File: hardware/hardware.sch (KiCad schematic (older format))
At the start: 39 parts, among them J1 USB_B_Micro, J2 Breakout, Q1 FS8205, U1 DW01+G, U2 TP4056, U3 USBLC6-2, U4 LM317A, U5 PIC18F45K50_QFP

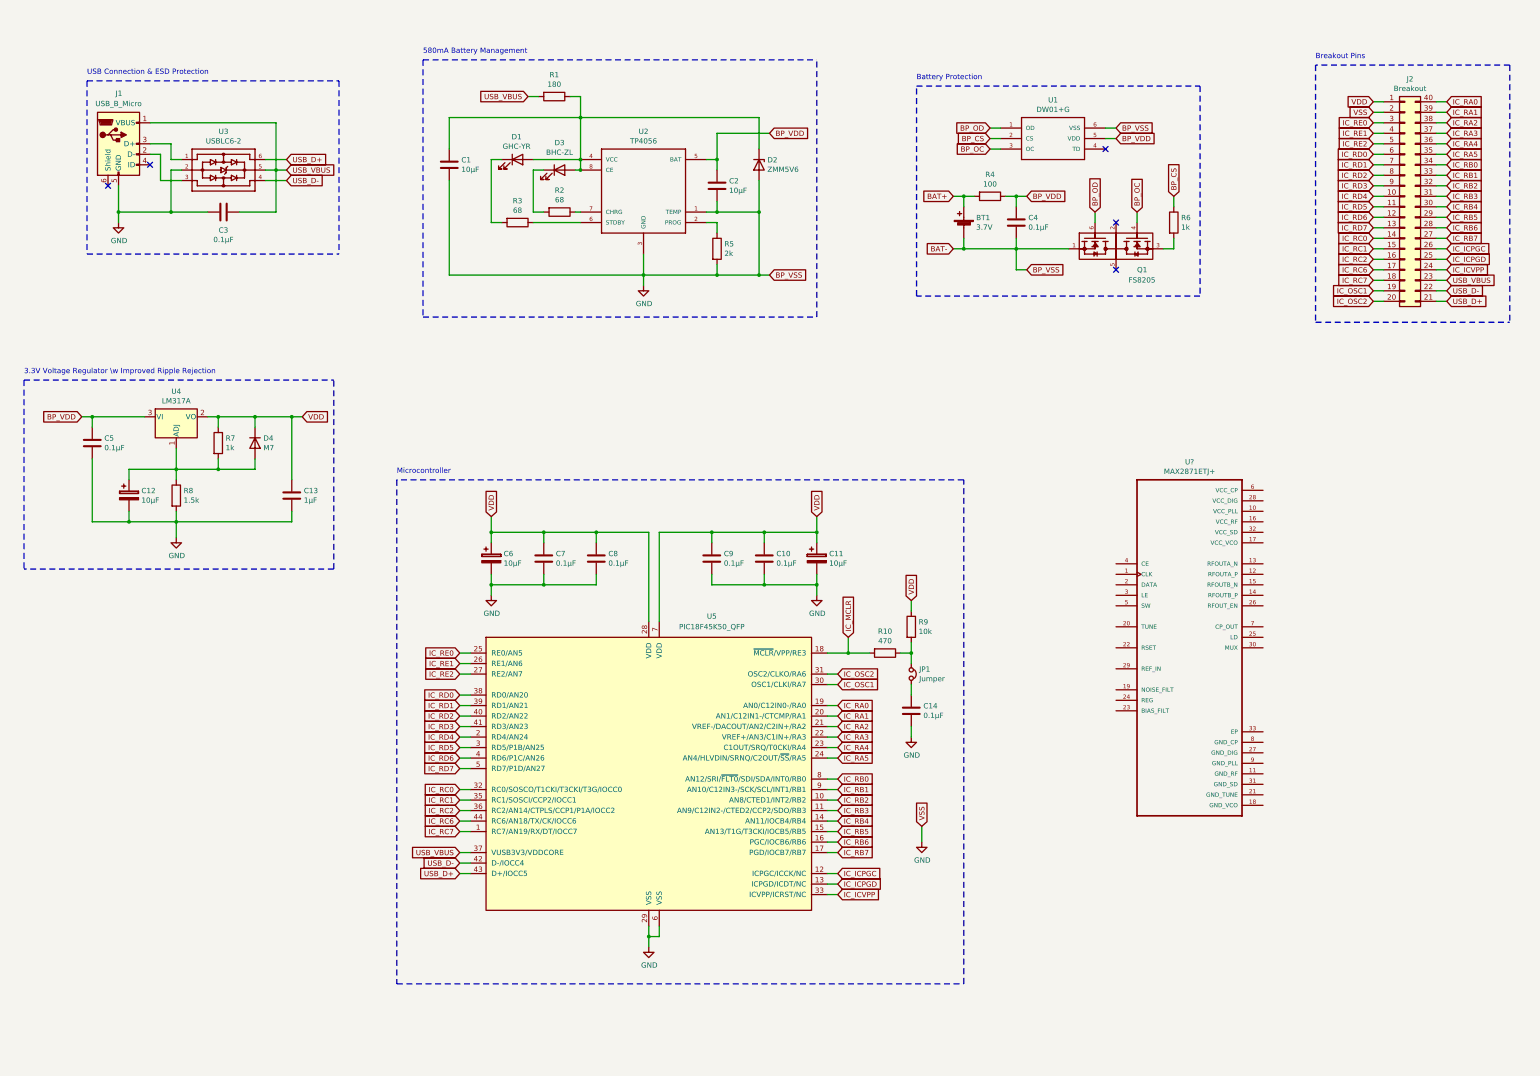
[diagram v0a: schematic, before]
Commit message: Compacted schematics.
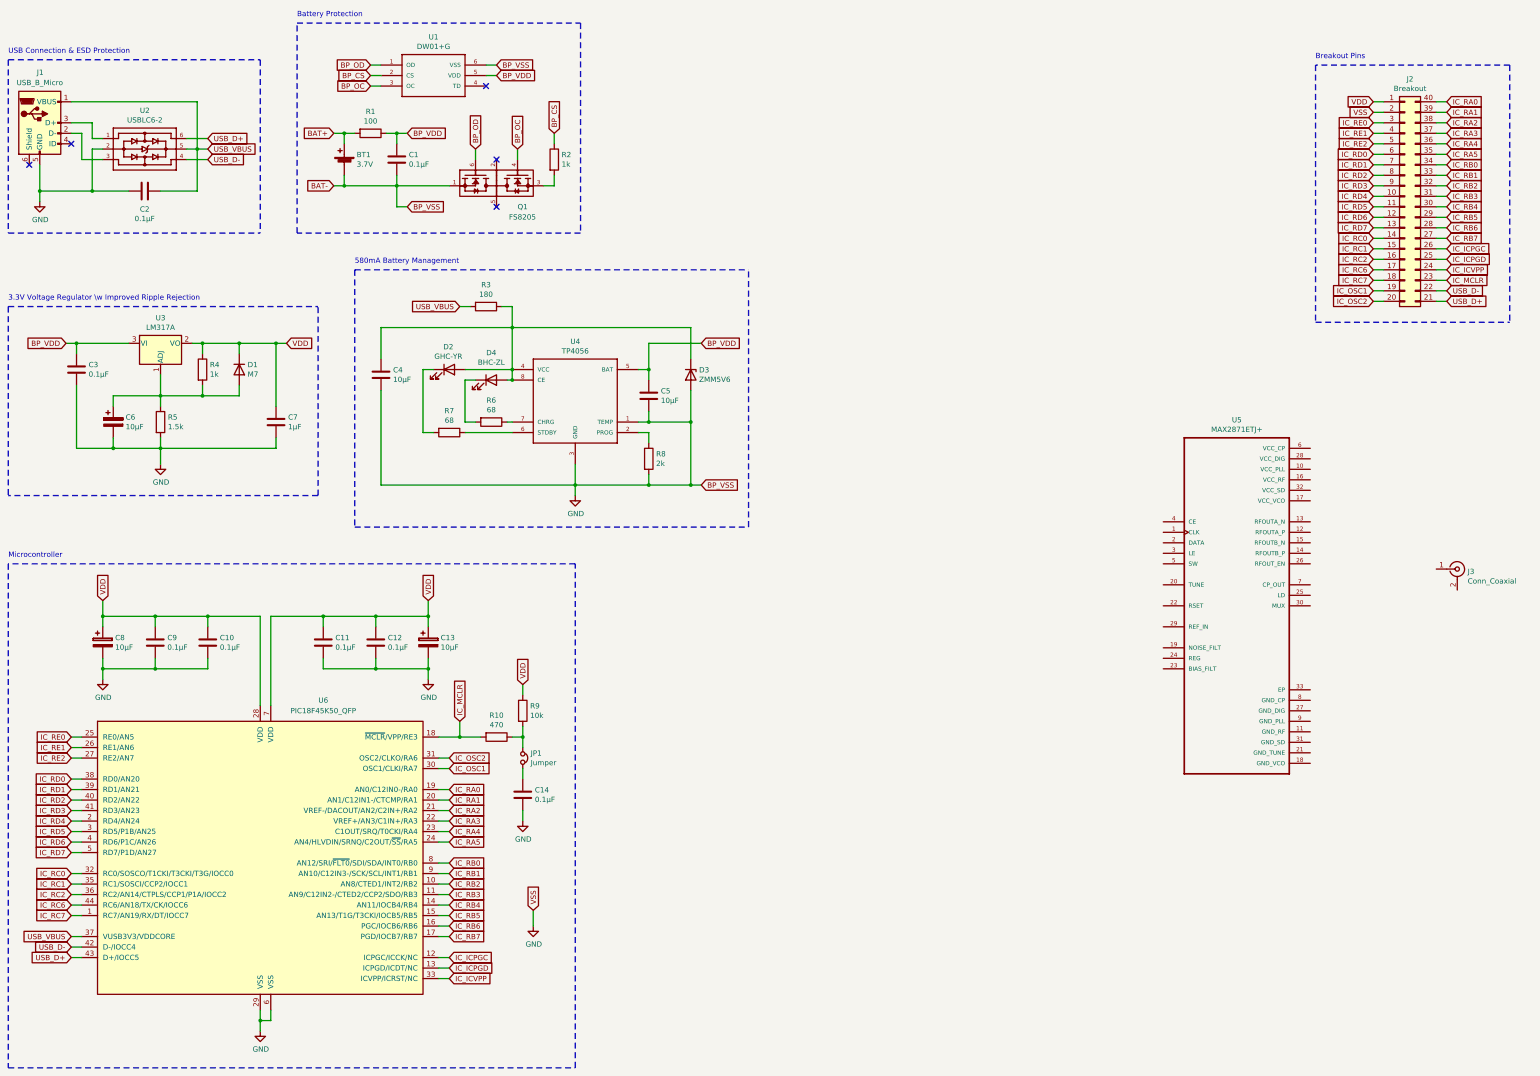
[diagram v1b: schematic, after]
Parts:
- added J3: Conn_Coaxial, symbol Connector:Conn_Coaxial
- gave numbers to parts that had none: 1
- renumbered C4 to C1, C8 to C10, C9 to C11, C10 to C12, C11 to C13, C3 to C2, C5 to C3, C1 to C4, C2 to C5, C12 to C6, C13 to C7, C6 to C8, C7 to C9, D4 to D1, D1 to D2, D2 to D3, D3 to D4, R4 to R1, R6 to R2, R1 to R3, R7 to R4, R8 to R5, R2 to R6, R3 to R7, R5 to R8, U3 to U2, U4 to U3, U2 to U4, U5 to U6
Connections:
- net IC_MCLR: now also J2.23 (Pin_23)
- net USB_VBUS: no longer J2.23 (Pin_23)
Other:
- moved on the sheet: BT1, C1, C10, C11, C12, C13, C14, C2, C3, C4, C5, C6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
